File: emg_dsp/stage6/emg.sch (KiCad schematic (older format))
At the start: 160 parts, among them U53 8X2X100, U54 VEE, U55 MIC5365-2.7, U56 AD7689, U57 GT12MABE, U58 LM828, U59 MIC5365-2.7, U60 74LVC1G, U61 TPS62410, U62 EN_VCC, U63 EN_VDD, U64 ABM10XTAL-16, U65 BF532-160, U66 ADSP_JTAG_CON, U67 NRF24L01, U68 74LCX541, U69 AT25DF041-MHF, U70 MAX6711Z, U71 TESTCON, U72 ANTENNA, U73 74LCX541, U74 74LCX541

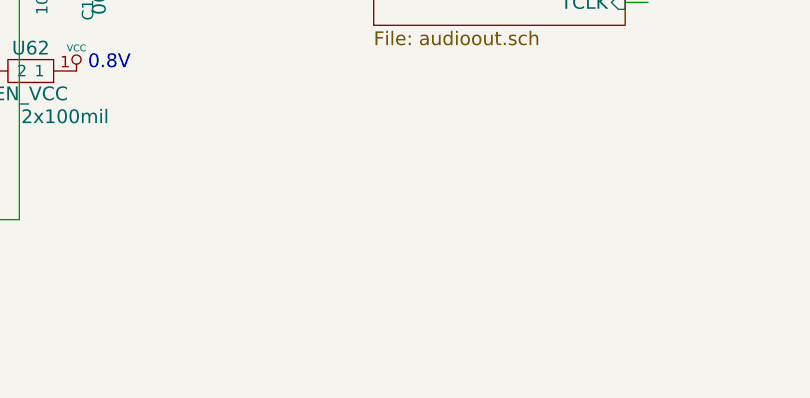
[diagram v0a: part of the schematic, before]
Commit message: board getting done! next up is silkscreen - pita.
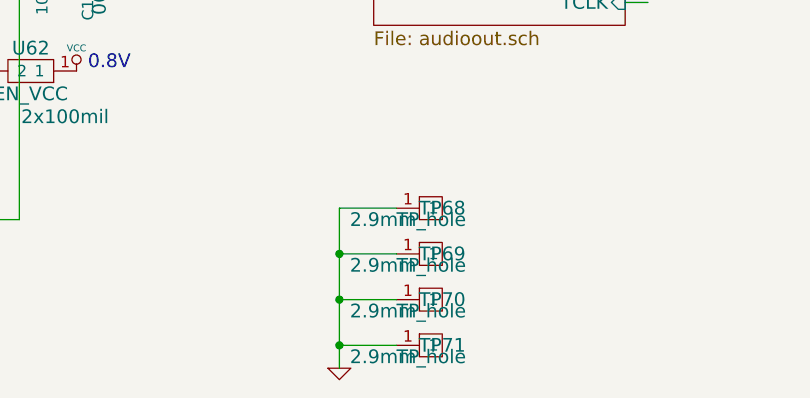
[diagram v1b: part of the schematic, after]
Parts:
- added TP68, TP69, TP70, TP71: TP, 2.9mm_hole, symbol TP
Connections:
- net GND: now also TP68.1, TP69.1, TP70.1, TP71.1
